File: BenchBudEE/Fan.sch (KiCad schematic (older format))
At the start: 0 parts

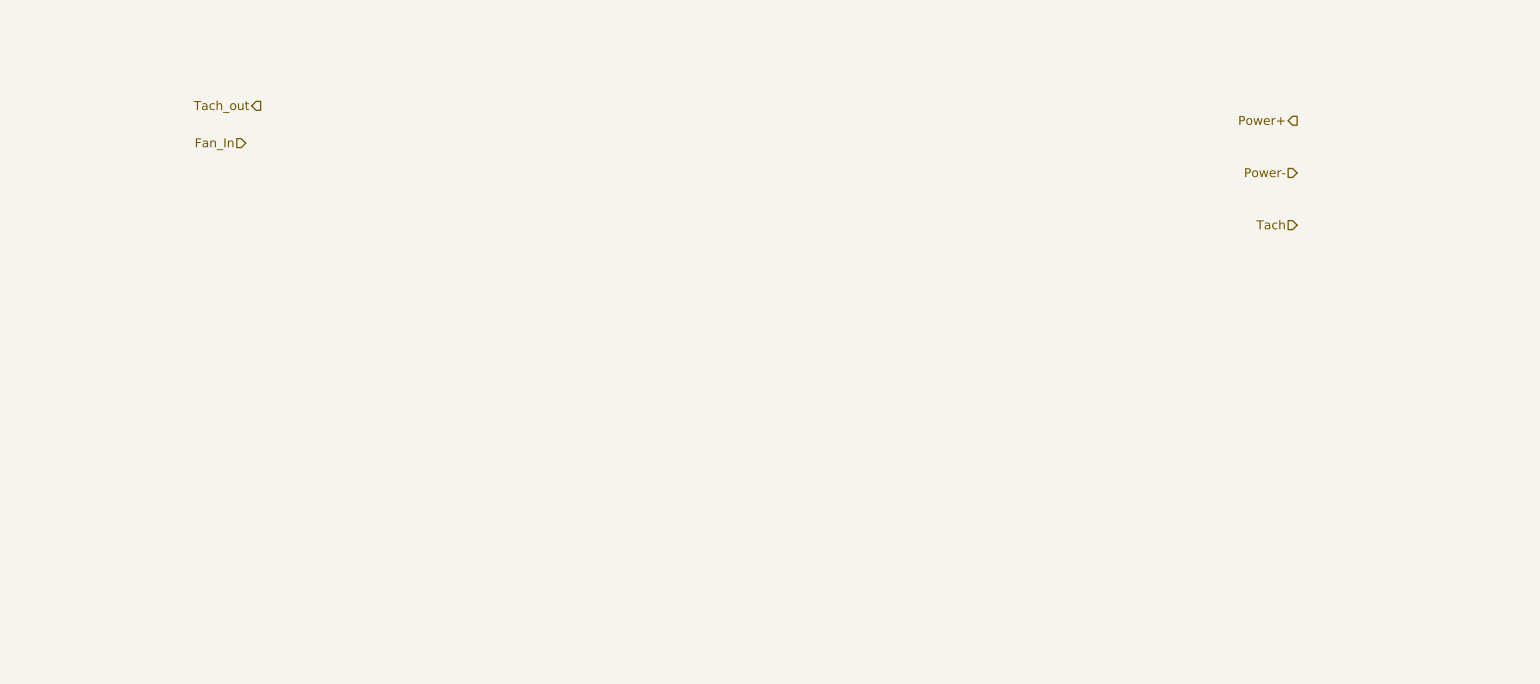
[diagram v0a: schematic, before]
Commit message: Fan driver block diagram
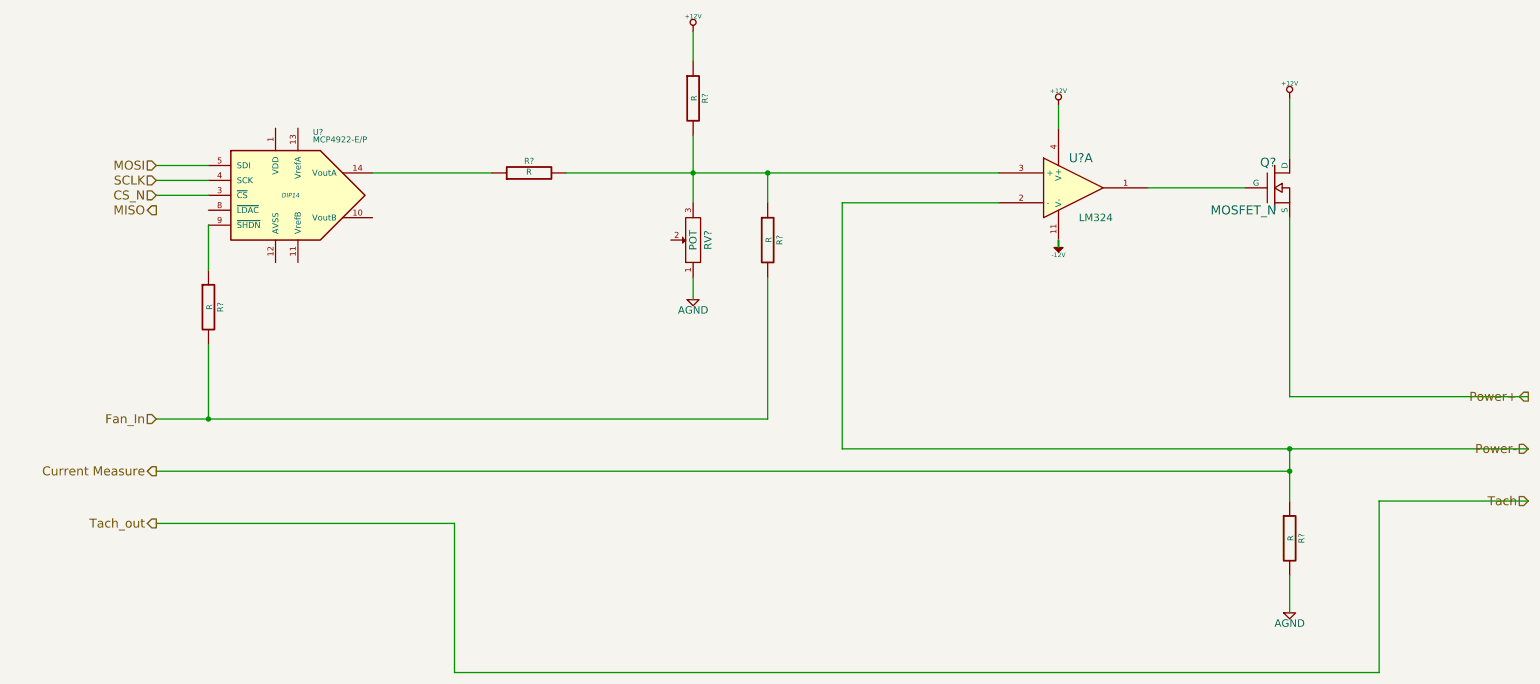
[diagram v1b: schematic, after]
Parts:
- added Q?: MOSFET_N, ~, symbol MOSFET_N
- added R? (x5): R, ~, symbol R
- added RV?: POT, ~, symbol POT
- added U?: LM324, symbol LM324
- added U?: MCP4922-E/P, DIP14, symbol MCP4922-E/P
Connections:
- net Fan_In: now also R?.2, R?.2
- net Power+: now also Q?.S
- new net: Q?.G, U?.1
- new net: R?.1, R?.2, R?.2, RV?.3, U?.3 (+)
- new net: R?.1, U?.14 (VoutA)
- new net: R?.1, U?.9 (~SHDN~)
- new net +12V: Q?.D, R?.1, U?.4 (V+)
- new net -12V: U?.11 (V-)
- new net AGND: R?.2, RV?.1
- new net CS_N: U?.3 (~CS~)
- new net Current Measure: R?.1, U?.2 (-)
- new net MOSI: U?.5 (SDI)
- new net SCLK: U?.4 (SCK)
